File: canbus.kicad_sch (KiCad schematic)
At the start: 12 parts, among them U1 MCP2562FD, U2 MCP2518FD, Y1 40 MHz

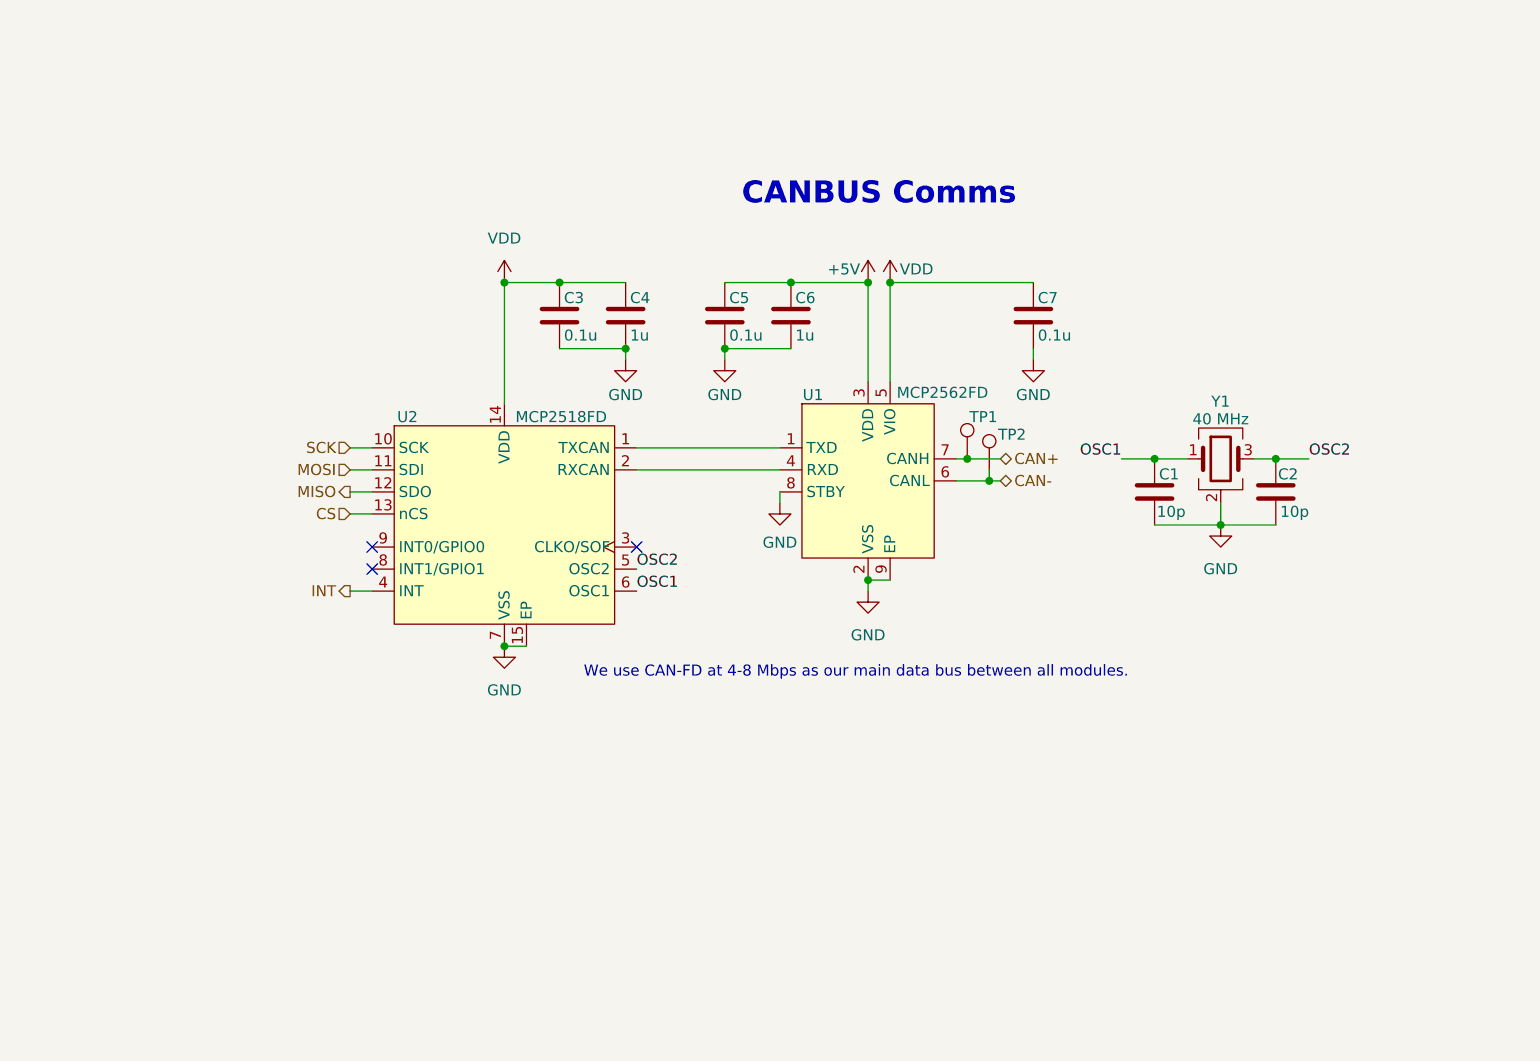
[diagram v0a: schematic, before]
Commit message: New v3.0 template
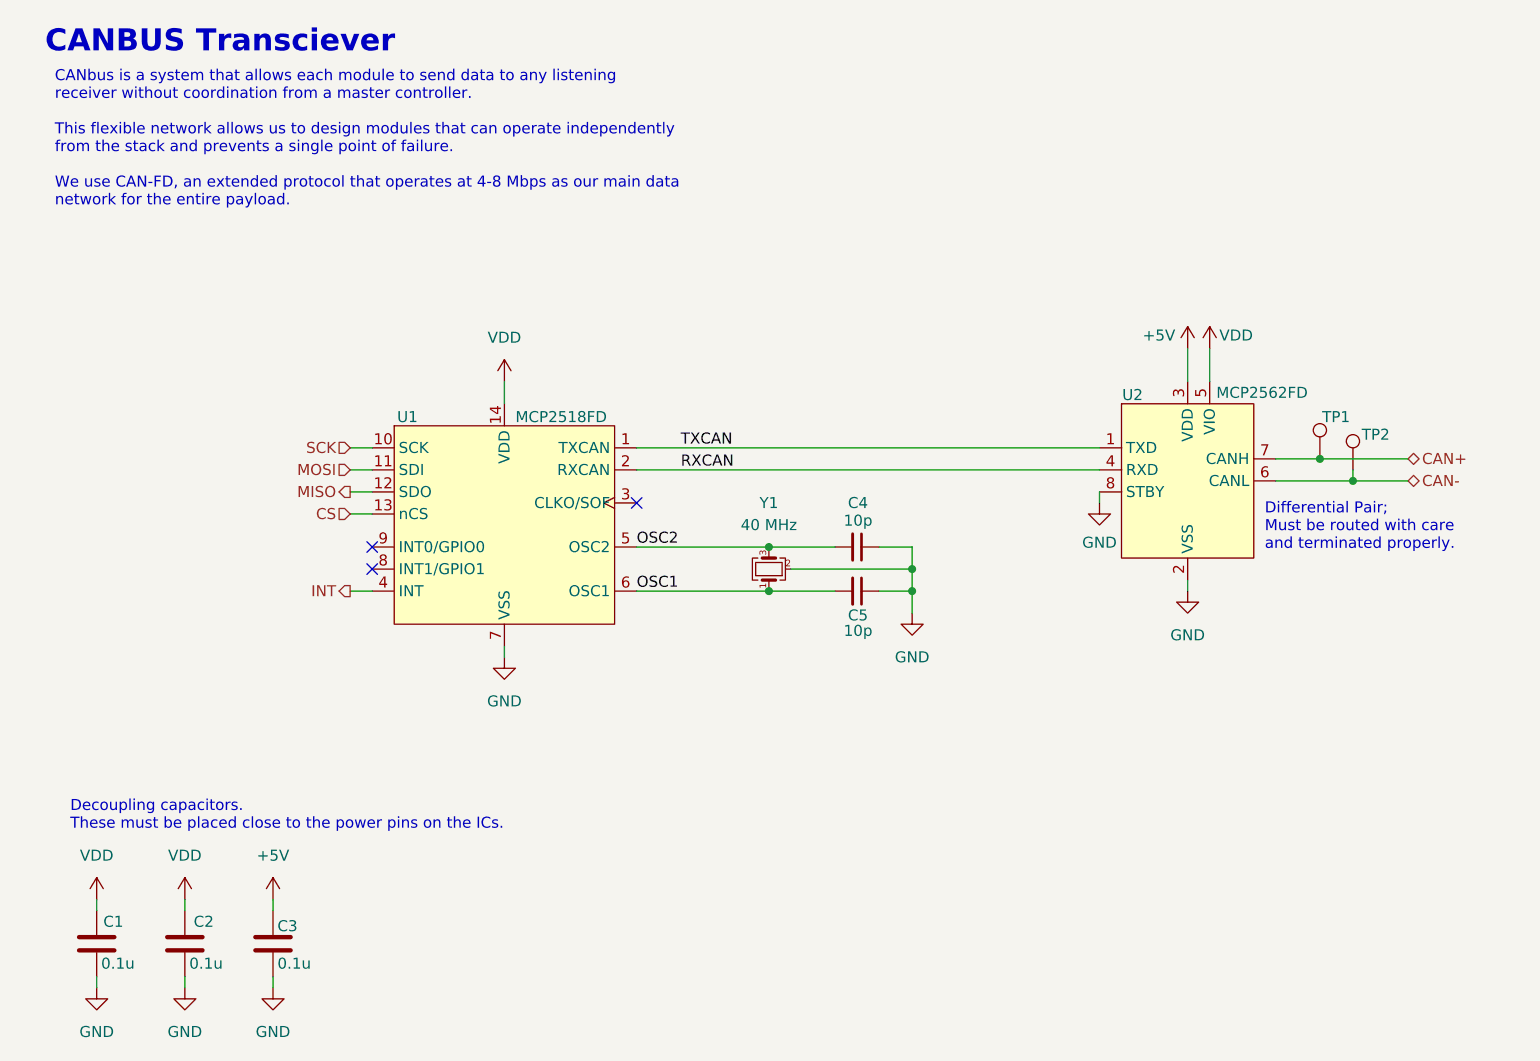
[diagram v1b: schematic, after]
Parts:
- removed C4, C6: 1u, Capacitor_SMD:C_0603_1608Metric, symbol Device:C
- removed C5, C7: 0.1u, Capacitor_SMD:C_0603_1608Metric, symbol Device:C
- added C1, C2: 0.1u, Capacitor_SMD:C_0805_2012Metric, symbol Device:C
- C3: footprint Capacitor_SMD:C_0603_1608Metric -> Capacitor_SMD:C_0805_2012Metric; Digikey 1276-CL10B104KB8NNNLCT-ND -> 1276-1003-1-ND; LCSC C913912 -> C1711; MPN CL10B104KB8NNNL -> CL21B104KBCNNNC
- C4: renamed from C2; footprint Capacitor_SMD:C_0603_1608Metric -> Capacitor_SMD:C_0805_2012Metric; symbol Device:C -> Device:C_Small; Digikey 1276-1027-1-ND -> 1276-2561-1-ND; LCSC C1634 -> C107107; MPN CL10C100JB8NNNC -> CL21C100CBANNNC
- C5: renamed from C1; footprint Capacitor_SMD:C_0603_1608Metric -> Capacitor_SMD:C_0805_2012Metric; symbol Device:C -> Device:C_Small; Digikey 1276-1027-1-ND -> 1276-2561-1-ND; LCSC C1634 -> C107107; MPN CL10C100JB8NNNC -> CL21C100CBANNNC
- TP1, TP2: now left out of the parts list
- U1: renamed from U2; Manufacturer Microchip Technology -> Microchip
- U2: renamed from U1; MPN MCP2562FDT-E/SN -> MCP2562FDT-H/SN; Manufacturer Microchip Technology -> Microchip
- Y1: symbol Device:Crystal_GND24 -> Device:Crystal_GND24_Small
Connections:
- net +5V: now also C3.1
- net GND: now also C1.2, C2.2; no longer U1.15 (EP), U2.9 (EP)
- net VDD: now also C1.1, C2.1; no longer C3.1
- net TXCAN: now reaches U1.1 (TXCAN), U2.1 (TXD)
- net RXCAN: now reaches U1.2 (RXCAN), U2.4 (RXD)
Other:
- note added: "CANBUS Transciever"
- note added: "CANbus is a system that allows each module to send data to any listening receiver without coordination from a master controller. This flexible network allows us to design modules that can operate independently from the stack and prevents a single point of failure. We use CAN-FD, an extended protocol that operates at 4-8 Mbps as our main data network for the entire payload."
- note added: "Decoupling capacitors. These must be placed close to the power pins on the ICs."
- note added: "Differential Pair; Must be routed with care and terminated properly."
- note removed: "CANBUS Comms"
- note removed: "We use CAN-FD at 4-8 Mbps as our main data bus between all modules."
- moved on the sheet: C4, C5, TP1, TP2
